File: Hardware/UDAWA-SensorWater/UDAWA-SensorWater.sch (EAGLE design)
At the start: 9 parts

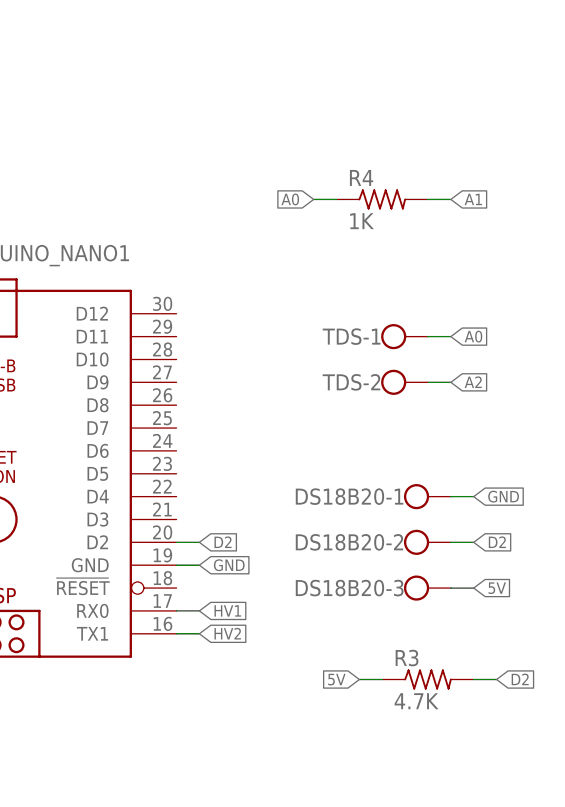
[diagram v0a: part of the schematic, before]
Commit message: First working version of Water Sensor
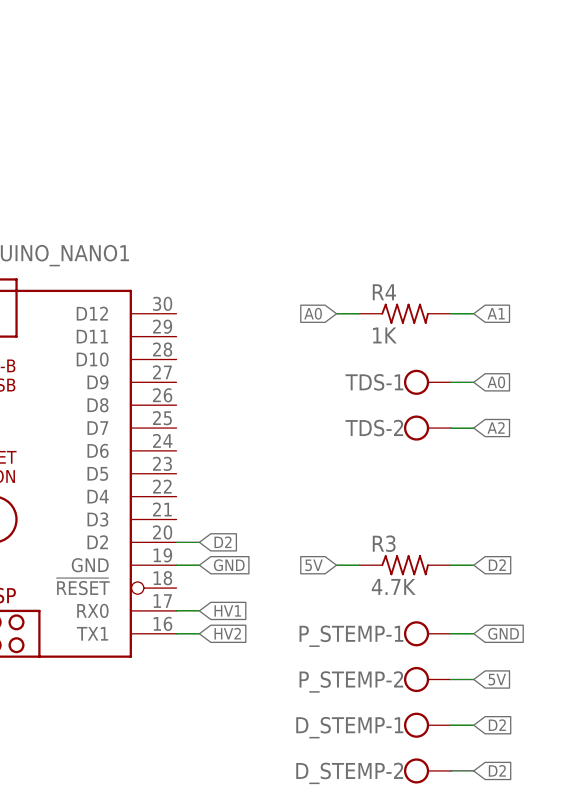
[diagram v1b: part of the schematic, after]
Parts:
- removed DS18B20: (no value), con-wago-500:W237-103
- added D_STEMP, P_STEMP: (no value), con-wago-500:W237-102
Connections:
- net 5V: now also P_STEMP-2.KL; no longer DS18B20-3.KL
- net D2: now also D_STEMP-1.KL, D_STEMP-2.KL; no longer DS18B20-2.KL
- net GND: now also P_STEMP-1.KL; no longer DS18B20-1.KL
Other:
- moved on the sheet: R3, R4, TDS-1, TDS-2
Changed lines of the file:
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@@
 </class>
 </classes>
+<groups>
+<schematic_group name="DS18B20"/>
+<schematic_group name="STDS"/>
+</groups>
 <parts>
 <part name="U$1" library="ESP32-DEVKITV1" deviceset="ESP32DEVKITV1" device=""/>
 <part name="HLK1" library="HLK-PM01" deviceset="HLK-PM01" device="3W"/>
-<part name="220V" library="con-wago-500" library_urn="urn:adsk.eagle:library:195" deviceset="W237-102" device="" package3d_urn="urn:adsk.eagle:package:10688/1"/>
+<part name="220V" library="con-wago-500" deviceset="W237-102" device="" package3d_urn="urn:adsk.eagle:package:10688/1"/>
 <part name="U$2" library="diy-modules" deviceset="LEVEL-SHIFTER-4CH" device=""/>
 <part name="ARDUINO_NANO1" library="ArduinoNanoV30" deviceset="ARDUINO_NANO" device=""/>
-<part name="TDS" library="con-wago-500" library_urn="urn:adsk.eagle:library:195" deviceset="W237-102" device="" package3d_urn="urn:adsk.eagle:package:10688/1"/>
-<part name="DS18B20" library="con-wago-500" library_urn="urn:adsk.eagle:library:195" deviceset="W237-103" device="" package3d_urn="urn:adsk.eagle:package:10691/1"/>
+<part name="TDS" library="con-wago-500" deviceset="W237-102" device="" package3d_urn="urn:adsk.eagle:package:10688/1"/>
 <part name="R3" library="rcl" library_urn="urn:adsk.eagle:library:334" deviceset="R-US_" device="0204/7" package3d_urn="urn:adsk.eagle:package:23498/2" value="4.7K"/>
 <part name="R4" library="rcl" library_urn="urn:adsk.eagle:library:334" deviceset="R-US_" device="0204/7" package3d_urn="urn:adsk.eagle:package:23498/2" value="1K"/>
+<part name="P_STEMP" library="con-wago-500" deviceset="W237-102" device="" package3d_urn="urn:adsk.eagle:package:10688/1"/>
+<part name="D_STEMP" library="con-wago-500" deviceset="W237-102" device="" package3d_urn="urn:adsk.eagle:package:10688/1"/>
 </parts>
 <sheets>
@@
 <attribute name="VALUE" x="-7.62" y="-5.08" size="1.778" layer="96" rot="R180"/>
 </instance>
-<instance part="TDS" gate="-1" x="20.32" y="-17.78" smashed="yes">
-<attribute name="NAME" x="20.32" y="-16.891" size="1.778" layer="95" rot="R180"/>
-</instance>
-<instance part="TDS" gate="-2" x="20.32" y="-22.86" smashed="yes">
-<attribute name="VALUE" x="17.78" y="-26.543" size="1.778" layer="96"/>
-<attribute name="NAME" x="20.32" y="-21.971" size="1.778" layer="95" rot="R180"/>
-</instance>
-<instance part="DS18B20" gate="-1" x="22.86" y="-35.56" smashed="yes">
-<attribute name="NAME" x="22.86" y="-34.671" size="1.778" layer="95" rot="R180"/>
-</instance>
-<instance part="DS18B20" gate="-2" x="22.86" y="-40.64" smashed="yes">
-<attribute name="NAME" x="22.86" y="-39.751" size="1.778" layer="95" rot="R180"/>
-</instance>
-<instance part="DS18B20" gate="-3" x="22.86" y="-45.72" smashed="yes">
-<attribute name="VALUE" x="20.32" y="-49.403" size="1.778" layer="96"/>
-<attribute name="NAME" x="22.86" y="-44.831" size="1.778" layer="95" rot="R180"/>
-</instance>
-<instance part="R3" gate="G$1" x="25.4" y="-55.88" smashed="yes">
-<attribute name="NAME" x="21.59" y="-54.3814" size="1.778" layer="95"/>
-<attribute name="VALUE" x="21.59" y="-59.182" size="1.778" layer="96"/>
-</instance>
-<instance part="R4" gate="G$1" x="20.32" y="-2.54" smashed="yes">
-<attribute name="NAME" x="16.51" y="-1.0414" size="1.778" layer="95"/>
-<attribute name="VALUE" x="16.51" y="-5.842" size="1.778" layer="96"/>
+<instance part="TDS" gate="-1" x="22.86" y="-22.86" smashed="yes" grouprefs="STDS">
+<attribute name="NAME" x="22.86" y="-21.971" size="1.778" layer="95" rot="R180"/>
+</instance>
+<instance part="TDS" gate="-2" x="22.86" y="-27.94" smashed="yes" grouprefs="STDS">
+<attribute name="VALUE" x="20.32" y="-31.623" size="1.778" layer="96"/>
+<attribute name="NAME" x="22.86" y="-27.051" size="1.778" layer="95" rot="R180"/>
+</instance>
+<instance part="R3" gate="G$1" x="22.86" y="-43.18" smashed="yes" grouprefs="DS18B20">
+<attribute name="NAME" x="19.05" y="-41.6814" size="1.778" layer="95"/>
+<attribute name="VALUE" x="19.05" y="-46.482" size="1.778" layer="96"/>
+</instance>
+<instance part="R4" gate="G$1" x="22.86" y="-15.24" smashed="yes" grouprefs="STDS">
+<attribute name="NAME" x="19.05" y="-13.7414" size="1.778" layer="95"/>
+<attribute name="VALUE" x="19.05" y="-18.542" size="1.778" layer="96"/>
+</instance>
+<instance part="P_STEMP" gate="-1" x="22.86" y="-50.8" smashed="yes" grouprefs="DS18B20">
+<attribute name="NAME" x="22.86" y="-49.911" size="1.778" layer="95" rot="R180"/>
+</instance>
+<instance part="P_STEMP" gate="-2" x="22.86" y="-55.88" smashed="yes" grouprefs="DS18B20">
+<attribute name="VALUE" x="20.32" y="-59.563" size="1.778" layer="96"/>
+<attribute name="NAME" x="22.86" y="-54.991" size="1.778" layer="95" rot="R180"/>
+</instance>
+<instance part="D_STEMP" gate="-1" x="22.86" y="-60.96" smashed="yes" grouprefs="DS18B20">
+<attribute name="NAME" x="22.86" y="-60.071" size="1.778" layer="95" rot="R180"/>
+</instance>
+<instance part="D_STEMP" gate="-2" x="22.86" y="-66.04" smashed="yes" grouprefs="DS18B20">
+<attribute name="VALUE" x="20.32" y="-69.723" size="1.778" layer="96"/>
+<attribute name="NAME" x="22.86" y="-65.151" size="1.778" layer="95" rot="R180"/>
 </instance>
 </instances>
@@
 </segment>
 <segment>
-<pinref part="DS18B20" gate="-1" pin="KL"/>
-<wire x1="27.94" y1="-35.56" x2="30.48" y2="-35.56" width="0.1524" layer="91"/>
-<label x="30.48" y="-35.56" size="1.27" layer="95" xref="yes"/>
+<pinref part="P_STEMP" gate="-1" pin="KL"/>
+<wire x1="27.94" y1="-50.8" x2="30.48" y2="-50.8" width="0.1524" layer="91" grouprefs="DS18B20"/>
+<label x="30.48" y="-50.8" size="1.27" layer="95" xref="yes" grouprefs="DS18B20"/>
 </segment>
 </net>
@@
 </segment>
 <segment>
-<pinref part="DS18B20" gate="-3" pin="KL"/>
-<wire x1="27.94" y1="-45.72" x2="30.48" y2="-45.72" width="0.1524" layer="91"/>
-<label x="30.48" y="-45.72" size="1.27" layer="95" xref="yes"/>
-</segment>
-<segment>
 <pinref part="R3" gate="G$1" pin="1"/>
-<wire x1="20.32" y1="-55.88" x2="17.78" y2="-55.88" width="0.1524" layer="91"/>
-<label x="17.78" y="-55.88" size="1.27" layer="95" rot="R180" xref="yes"/>
+<wire x1="17.78" y1="-43.18" x2="15.24" y2="-43.18" width="0.1524" layer="91" grouprefs="DS18B20"/>
+<label x="15.24" y="-43.18" size="1.27" layer="95" rot="R180" xref="yes" grouprefs="DS18B20"/>
+</segment>
+<segment>
+<pinref part="P_STEMP" gate="-2" pin="KL"/>
+<wire x1="27.94" y1="-55.88" x2="30.48" y2="-55.88" width="0.1524" layer="91" grouprefs="DS18B20"/>
+<label x="30.48" y="-55.88" size="1.27" layer="95" xref="yes" grouprefs="DS18B20"/>
 </segment>
 </net>
@@
 <segment>
 <pinref part="TDS" gate="-1" pin="KL"/>
-<wire x1="25.4" y1="-17.78" x2="27.94" y2="-17.78" width="0.1524" layer="91"/>
-<label x="27.94" y="-17.78" size="1.27" layer="95" xref="yes"/>
+<wire x1="27.94" y1="-22.86" x2="30.48" y2="-22.86" width="0.1524" layer="91" grouprefs="STDS"/>
+<label x="30.48" y="-22.86" size="1.27" layer="95" xref="yes" grouprefs="STDS"/>
 </segment>
 <segment>
@@
 <segment>
 <pinref part="R4" gate="G$1" pin="1"/>
-<wire x1="15.24" y1="-2.54" x2="12.7" y2="-2.54" width="0.1524" layer="91"/>
-<label x="12.7" y="-2.54" size="1.27" layer="95" rot="R180" xref="yes"/>
+<wire x1="17.78" y1="-15.24" x2="15.24" y2="-15.24" width="0.1524" layer="91" grouprefs="STDS"/>
+<label x="15.24" y="-15.24" size="1.27" layer="95" rot="R180" xref="yes" grouprefs="STDS"/>
 </segment>
 </net>
@@
 <segment>
 <pinref part="TDS" gate="-2" pin="KL"/>
-<wire x1="25.4" y1="-22.86" x2="27.94" y2="-22.86" width="0.1524" layer="91"/>
-<label x="27.94" y="-22.86" size="1.27" layer="95" xref="yes"/>
+<wire x1="27.94" y1="-27.94" x2="30.48" y2="-27.94" width="0.1524" layer="91" grouprefs="STDS"/>
+<label x="30.48" y="-27.94" size="1.27" layer="95" xref="yes" grouprefs="STDS"/>
 </segment>
 <segment>
@@
 <net name="D2" class="0">
 <segment>
-<pinref part="DS18B20" gate="-2" pin="KL"/>
-<wire x1="27.94" y1="-40.64" x2="30.48" y2="-40.64" width="0.1524" layer="91"/>
-<label x="30.48" y="-40.64" size="1.27" layer="95" xref="yes"/>
-</segment>
-<segment>
 <pinref part="ARDUINO_NANO1" gate="G$1" pin="D2"/>
 <wire x1="-2.54" y1="-40.64" x2="0" y2="-40.64" width="0.1524" layer="91"/>
@@
 <segment>
 <pinref part="R3" gate="G$1" pin="2"/>
-<wire x1="30.48" y1="-55.88" x2="33.02" y2="-55.88" width="0.1524" layer="91"/>
-<label x="33.02" y="-55.88" size="1.27" layer="95" xref="yes"/>
+<wire x1="27.94" y1="-43.18" x2="30.48" y2="-43.18" width="0.1524" layer="91" grouprefs="DS18B20"/>
+<label x="30.48" y="-43.18" size="1.27" layer="95" xref="yes" grouprefs="DS18B20"/>
+</segment>
+<segment>
+<pinref part="D_STEMP" gate="-1" pin="KL"/>
+<wire x1="27.94" y1="-60.96" x2="30.48" y2="-60.96" width="0.1524" layer="91" grouprefs="DS18B20"/>
+<label x="30.48" y="-60.96" size="1.27" layer="95" xref="yes" grouprefs="DS18B20"/>
+</segment>
+<segment>
+<pinref part="D_STEMP" gate="-2" pin="KL"/>
+<wire x1="27.94" y1="-66.04" x2="30.48" y2="-66.04" width="0.1524" layer="91" grouprefs="DS18B20"/>
+<label x="30.48" y="-66.04" size="1.27" layer="95" xref="yes" grouprefs="DS18B20"/>
 </segment>
 </net>
@@
 <segment>
 <pinref part="R4" gate="G$1" pin="2"/>
-<wire x1="25.4" y1="-2.54" x2="27.94" y2="-2.54" width="0.1524" layer="91"/>
-<label x="27.94" y="-2.54" size="1.27" layer="95" xref="yes"/>
+<wire x1="27.94" y1="-15.24" x2="30.48" y2="-15.24" width="0.1524" layer="91" grouprefs="STDS"/>
+<label x="30.48" y="-15.24" size="1.27" layer="95" xref="yes" grouprefs="STDS"/>
 </segment>
 </net>
@@
 packages will not be understood (or retained) with this version.
 </note>
+<note version="9.5" severity="warning">
+Since Version 9.5, EAGLE supports persistent groups with
+schematics, and board files. Those persistent groups
+will not be understood (or retained) with this version.
+</note>
 <note version="8.4" severity="warning">
